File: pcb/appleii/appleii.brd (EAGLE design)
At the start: 75 x 47 mm, 17 parts, among them J1 POWER_JACKPTH, J2 ATX24RH

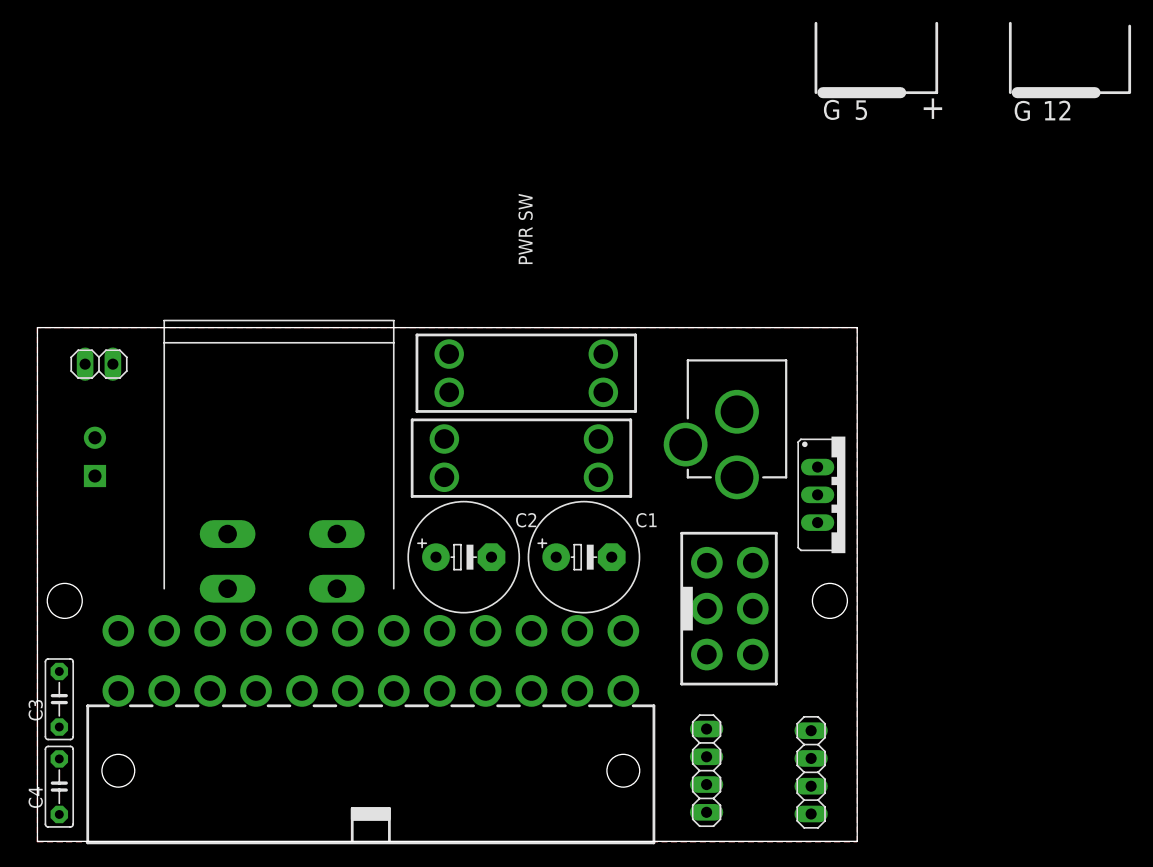
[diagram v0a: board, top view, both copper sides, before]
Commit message: working on appleii
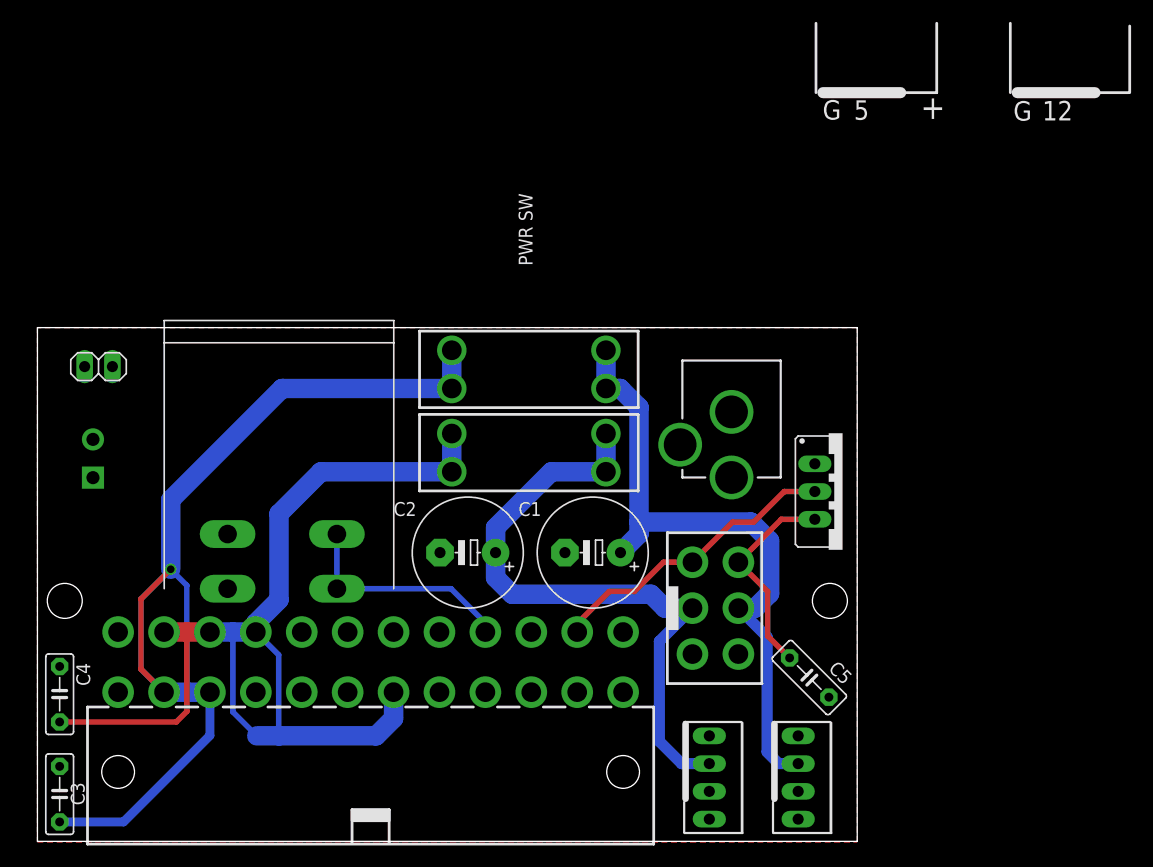
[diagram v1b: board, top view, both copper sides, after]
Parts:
- removed JP3: (no value), atx_power_control:1X04
- added C5: (no value), capacitor-wima:C5B2.5
- added JP4: (no value), appleii:1X04
- JP1: device atx_power_control:1X04 -> appleii:1X04
- moved C3 8.68 mm to (2.03, 4.32)
- moved C4 8.46 mm to (2.03, 13.5)
- moved JP1 8.40 mm to (69.6, 5.84)
- moved U$4 1.32 mm to (62.0, 21.3)
- moved C1 0.90 mm to (50.8, 26.4), turned to 180 degrees
- moved U$8 0.84 mm to (45.0, 35.6)
- moved C2 0.56 mm to (39.4, 26.4), turned to 180 degrees
- moved J1 0.50 mm to (63.5, 47.0)
- moved U$2 0.42 mm to (45.0, 43.2)
- moved IC1 0.40 mm to (73.7, 32.0)
- moved J7 0.24 mm to (5.08, 33.3)
- moved JP2 0.23 mm to (5.59, 43.4)
- moved J2 0.11 mm to (30.5, 8.89)
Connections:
- net +12V: now also C1.+, JP1.2; no longer JP1.3
- net +5V: now also C2.+, JP4.2; no longer JP3.3
- net -5V: now also C5.1
- net GND: now also C1.-, C2.-, C3.2, C4.2, C5.2, JP1.1, JP4.1; no longer JP1.4, JP3.4
- net N$6: now also C4.1
- net N$8: now also C3.1
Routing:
- net N$8: track 0.00 -> 103.3 mm, vias 0 -> 1
- net N$6: track 0.00 -> 96.7 mm
- net +12V: track 0.00 -> 60.2 mm
- net +5V: track 0.00 -> 58.3 mm
- net -12V: track 0.00 -> 27.5 mm
- net N$5: track 0.00 -> 20.7 mm
- net -5V: track 0.00 -> 19.3 mm
